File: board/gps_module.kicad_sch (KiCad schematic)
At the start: 18 parts, among them IC1 RT9193-33GB, J5 Conn_Coaxial, U6 NEO-M7N, U7 MAX2679B

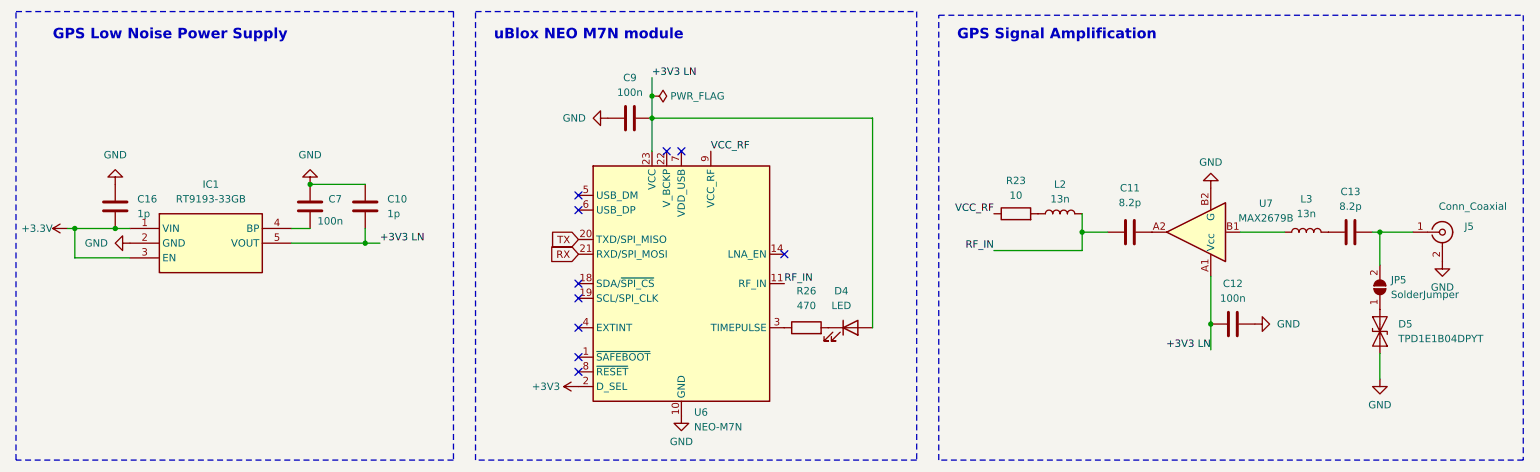
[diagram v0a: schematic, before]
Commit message: Started work on PCB design, more work on rewritting firmware to be semi usable
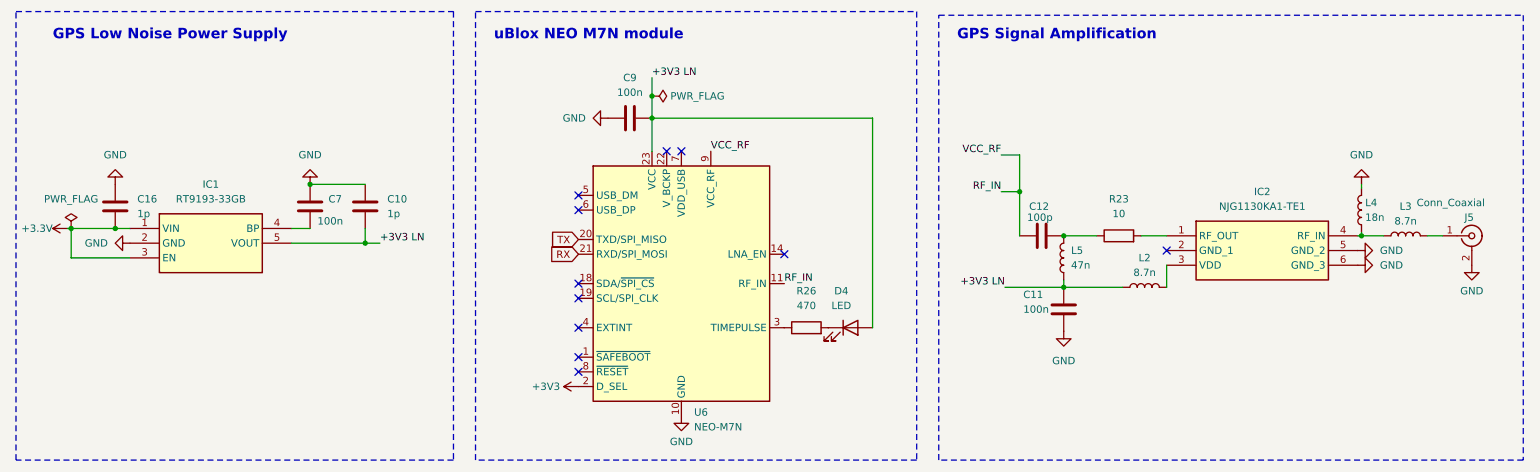
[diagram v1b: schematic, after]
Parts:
- removed C13: 8.2p, Capacitor_SMD:C_0603_1608Metric, symbol Device:C
- removed D5: TPD1E1B04DPYT, Imported_Footprints:DPY_R-PX1SON-N2_, symbol Imported_Symbols:TPD1E1B04DPYT
- removed JP5: SolderJumper, Jumper:SolderJumper-2_P1.3mm_Open_Pad1.0x1.5mm, symbol Jumper:SolderJumper_2_Open
- removed U7: MAX2679B, Package_BGA:WLP-4_0.83x0.83mm_P0.4mm, symbol RF_Amplifier:MAX2679B
- added IC2: NJG1130KA1-TE1, Imported_Footprints:SOTFL50P160X60-6N, symbol Imported_Symbols:NJG1130KA1-TE1
- added L4: 18n, Inductor_SMD:L_0805_2012Metric, symbol Device:L
- added L5: 47n, Inductor_SMD:L_0603_1608Metric, symbol Device:L
- C11: value 8.2p -> 100n
- C12: value 100n -> 100p
- L2, L3: value 13n -> 8.7n; footprint Inductor_SMD:L_0402_1005Metric -> Inductor_SMD:L_0603_1608Metric
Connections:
- net +3V3 LN: now also C11.1, L2.1, L5.1; no longer C12.2
- net GND: now also C11.2, IC2.5 (GND_2), IC2.6 (GND_3), L4.2; no longer C12.1
- net RF_IN: now also C12.1, U6.9 (VCC_RF); no longer C11.1, L2.2
- net at L3.2: now also J5.1 (In)
- net at L3.1: now also IC2.4 (RF_IN), L4.1
- net at R23.2: now also IC2.1 (RF_OUT); no longer L2.1
- net VCC_RF: no longer names the net of R23.1
- net VCC_RF: now also C12.2, L5.2; no longer U6.9 (VCC_RF)
- new net: IC2.3 (VDD), L2.2
- no-connect marks 10 -> 11
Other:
- moved on the sheet: J5, L3
